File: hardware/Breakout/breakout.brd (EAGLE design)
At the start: 100 x 80 mm, 14 parts, among them IC1 24AA04SN, IC2 MAX490CSA, X1 VISCA

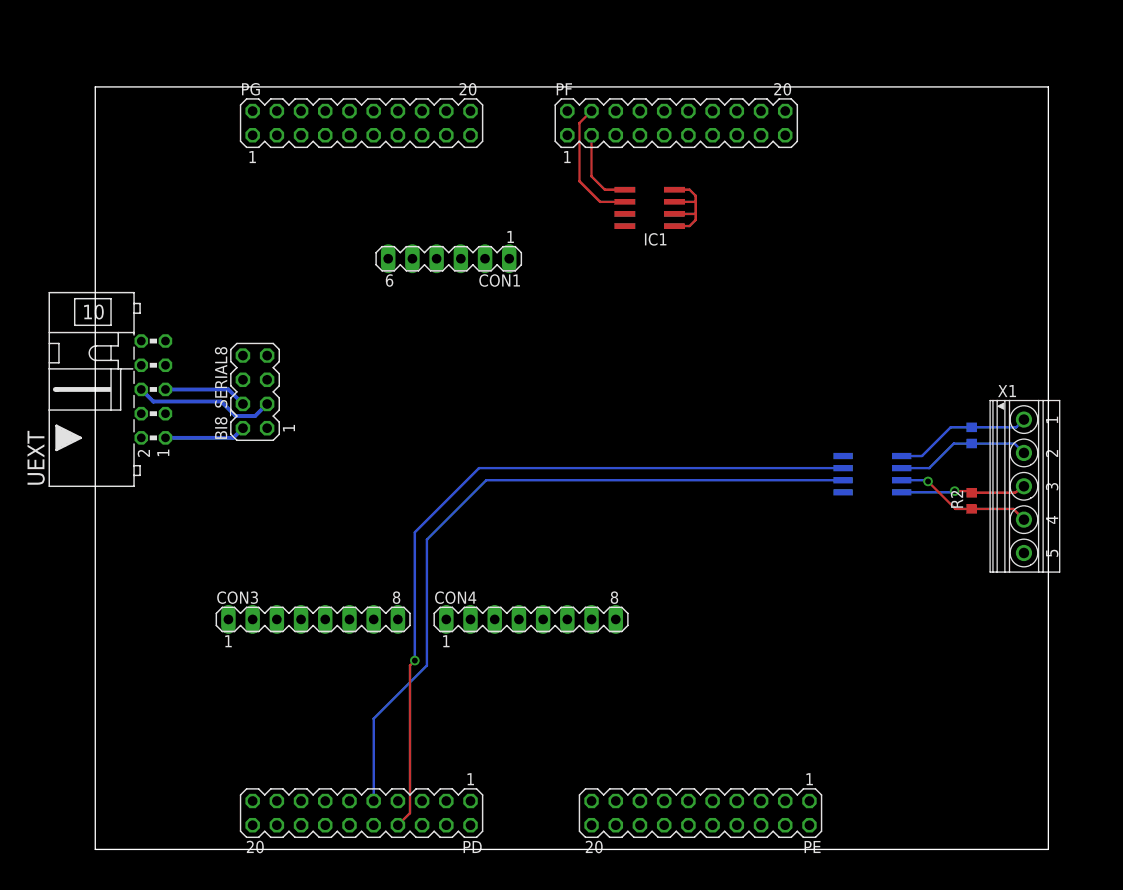
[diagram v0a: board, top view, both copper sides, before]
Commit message: Breakout Board v1
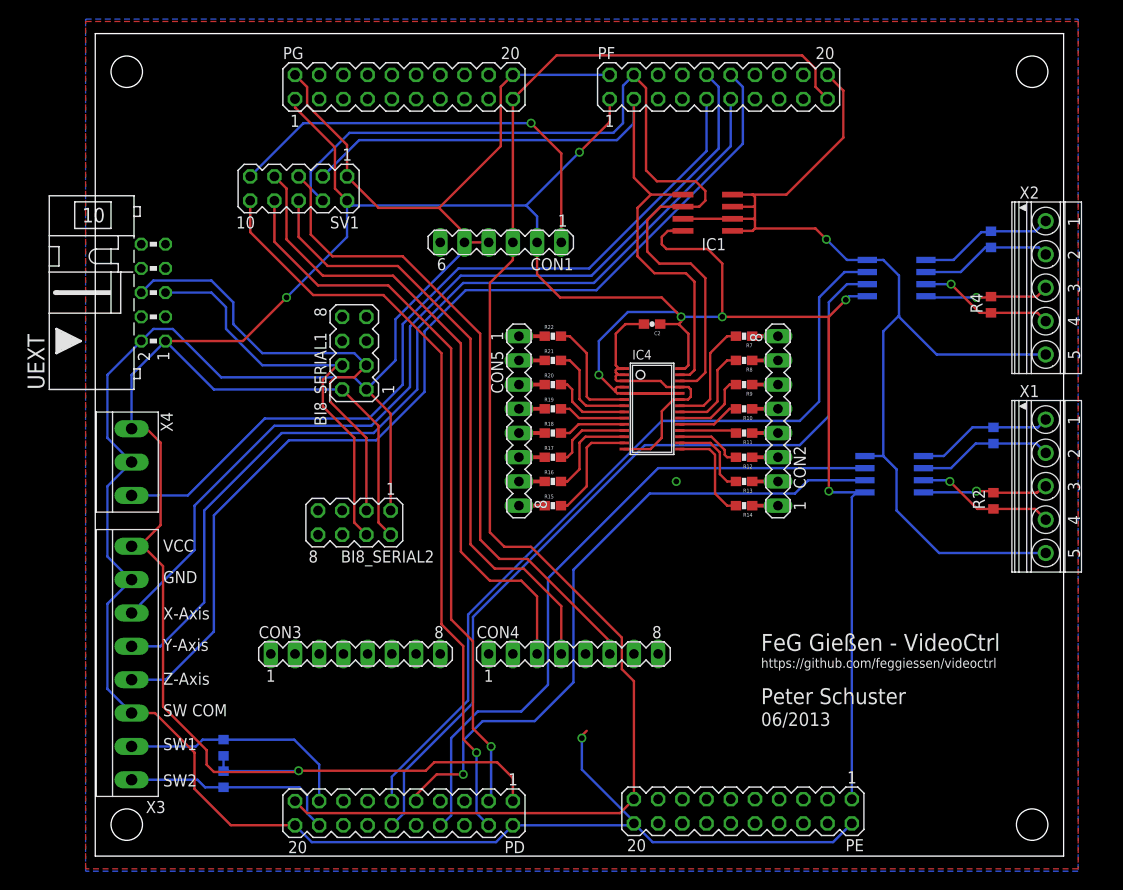
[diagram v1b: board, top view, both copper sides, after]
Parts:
- removed BI8_SERIAL: (no value), con-lstb:MA04-2
- added BI8_SERIAL1, BI8_SERIAL2: (no value), con-lstb:MA04-2
- added C2: 100nF, SparkFun:0603-CAP
- added CON2: LED2, con-lstb:MA08-1
- added CON5: LED1, con-lstb:MA08-1
- added IC3: MAX490CSA, maxim:SO08
- added IC4: PCA9685, wsmith:TSSOP28
- added R10, R11, R12, R13, R14, R15, R16, R17, R18, R19, R20, R21, R22, R7, R8, R9: 180, SparkFun:0603-RES
- added R3, R4: 120, resistor:R0603
- added R5, R6: 10K, resistor:R0603
- added SV1: DISPLAY, con-lstb:MA05-2
- added X2: RS485, con-phoenix-350:1751277
- added X3: JOYSTICK, con-ria-59:8POL35
- added X4: SLIDER, con-ria-59:3POL35
- moved UEXT 10.2 mm to (6.10, 58.4)
- moved IC1 6.12 mm to (64.3, 66.8)
- moved PG 5.85 mm to (32.4, 80.0)
- moved PF 5.84 mm to (65.4, 80.0)
- moved CON3 5.73 mm to (27.3, 20.5)
- moved CON4 5.73 mm to (50.2, 20.5)
- moved CON1 5.72 mm to (42.5, 63.7)
- moved PE 4.45 mm to (67.9, 4.00)
- moved PD 4.45 mm to (32.4, 3.80)
- moved R1 2.29 mm to (94.2, 43.4)
- moved R2 2.29 mm to (94.2, 36.6)
- moved X1 2.29 mm to (99.8, 38.1)
- moved IC2 2.29 mm to (83.8, 39.4)
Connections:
- new net L0: CON5.1, R22.1
- new net L1: CON5.2, R21.1
- new net L10: CON2.3, R12.1
- new net L11: CON2.4, R11.1
- new net L12: CON2.5, R10.1
- new net L13: CON2.6, R9.1
- new net L14: CON2.7, R8.1
- new net L15: CON2.8, R7.1
- new net L2: CON5.3, R20.1
- new net L3: CON5.4, R19.1
- new net L4: CON5.5, R18.1
- new net L5: CON5.6, R17.1
- new net L6: CON5.7, R16.1
- new net L7: CON5.8, R15.1
- new net L8: CON2.1, R14.1
- new net L9: CON2.2, R13.1
- new net N$10: IC4.9, R19.2
- new net N$11: IC4.8, R20.2
- new net N$12: IC4.7, R21.2
- new net N$19: IC4.6, R22.2
- new net N$20: IC4.15, R14.2
- new net N$21: IC4.16, R13.2
- new net N$22: IC4.17, R12.2
- new net N$23: IC4.18, R11.2
- new net N$24: IC4.19, R10.2
- new net N$25: IC4.20, R9.2
- new net N$26: IC4.21, R8.2
- new net N$27: IC4.22, R7.2
- new net N$4: IC4.13, R15.2
- new net N$5: IC4.12, R16.2
- new net N$7: IC4.11, R17.2
- new net N$9: IC4.10, R18.2
- new net PD0/DISP_MODE: PD.3, SV1.8
- new net PD1/ENC_INT: PD.4, SV1.10
- new net PD10: PD.13
- new net PD11: PD.14
- new net PD12: PD.15
- new net PD13: PD.16
- new net PD14/JOY_T1: PD.17, R5.2, X3.7
- new net PD15/JOY_T2: PD.18, R6.2, X3.8
- new net PD3: PD.6
- new net PD4: PD.7
- new net PD7: PD.10
- new net PE0: PE.3
- new net PE1: PE.4
- new net PE10: PE.13
- new net PE11: PE.14
- new net PE12: PE.15
- new net PE13: PE.16
- new net PE14: PE.17
- new net PE15: PE.18
- new net PE2: PE.5
- new net PE3: PE.6
- new net PE4: PE.7
- new net PE5: PE.8
- new net PE6: PE.9
- new net PE7: PE.10
- new net PE8: PE.11
- new net PE9: PE.12
- new net PF12: PF.15
- new net PF13: PF.16
- new net PF14: PF.17
- new net PF15: PF.18
- new net PF2: PF.5
- new net PF3: PF.6
- new net PF4: PF.7
- new net PF5: PF.8
- new net PG0: PG.3
- new net PG1: PG.4
- new net PG12: PG.15
- new net PG15: PG.18
- new net PG2: PG.5
- new net PG3: PG.6
- new net PG4: PG.7
- new net PG5: PG.8
- new net PG6: PG.9
- new net PG7: PG.10
- new net PG8: PG.11
- new net PG9: PG.12
- new net RS485_RXD_N: IC3.7, R4.1, X2.4
- new net RS485_RXD_P: IC3.8, R4.2, X2.3
- new net RS485_TXD_N: IC3.6, R3.1, X2.2
- new net RS485_TXD_P: IC3.5, R3.2, X2.1
- net A1: now also X4.3
- net A2: now also X3.3
- net A3: now also X3.4
- net A4: now also X3.5
- net GND: now also BI8_SERIAL1.1, BI8_SERIAL2.1, C2.2, IC3.4, IC4.1, IC4.14, IC4.2, IC4.23, IC4.25, IC4.3, SV1.1, X2.5, X3.2, X3.6, X4.2; no longer BI8_SERIAL.1
- net I2C1_SCL: now also BI8_SERIAL1.4, BI8_SERIAL2.4; no longer BI8_SERIAL.4
- net I2C1_SDA: now also BI8_SERIAL1.3, BI8_SERIAL2.3; no longer BI8_SERIAL.3
- net I2C2_SCL: now also IC4.26, SV1.4
- net I2C2_SDA: now also IC4.27, SV1.3
- net RST: now also SV1.9
- net SPI1_MOSI: now also SV1.6
- net SPI1_NSS: now also SV1.7
- net SPI1_SCK: now also SV1.5
- net USART3_RX: now also IC3.2
- net USART3_TX: now also IC3.3
- net VCC: now also BI8_SERIAL1.2, BI8_SERIAL2.2, C2.1, IC3.1, IC4.24, IC4.28, IC4.4, IC4.5, R5.1, R6.1, SV1.2, X3.1, X4.1; no longer BI8_SERIAL.2
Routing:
- net GND: track 12.0 -> 410.3 mm, vias 0 -> 3
- net VCC: track 8.55 -> 368.1 mm, vias 0 -> 8
- net +5V: track 0.00 -> 157.0 mm
- net A4: track 0.00 -> 106.0 mm
- net A3: track 0.00 -> 98.9 mm
- net A2: track 0.00 -> 96.5 mm
- net USART3_RX: track 0.00 -> 88.2 mm
- net USART3_TX: track 0.00 -> 86.1 mm
- net A1: track 0.00 -> 84.5 mm
- net PD1/ENC_INT: track 0.00 -> 80.2 mm, vias 0 -> 1
- net I2C2_SCL: track 13.6 -> 93.1 mm
- net PD0/DISP_MODE: track 0.00 -> 76.8 mm, vias 0 -> 1
- net SPI1_SCK: track 0.00 -> 69.6 mm
- net I2C2_SDA: track 8.39 -> 76.7 mm
- net SPI1_NSS: track 0.00 -> 67.8 mm
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- added copper zone on layer 1, net GND
- added copper zone on layer 16, net GND
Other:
- board size 100 x 80 mm -> 101.6 x 86.3 mm
- board text added: "06/2013"
- board text added: "FeG Gießen - VideoCtrl"
- board text added: "GND"
- board text added: "Peter Schuster"
- board text added: "SW COM"
- board text added: "SW1"
- board text added: "SW2"
- board text added: "VCC"
- board text added: "X-Axis"
- board text added: "Y-Axis"
- board text added: "Z-Axis"
- board text added: "https://github.com/feggiessen/videoctrl"
